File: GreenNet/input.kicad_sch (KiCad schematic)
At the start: 74 parts, among them Q3 IRF9358TRPBF, Q4 SI3932DV-T1-GE3, Q5 SI3993CDV-T1-GE3, U2 USB_C_Receptacle_12P, U3 USB_C_Receptacle_12P, U4 CP2102N-A02-GQFN28, U6 CYPD3177-24LQXQT

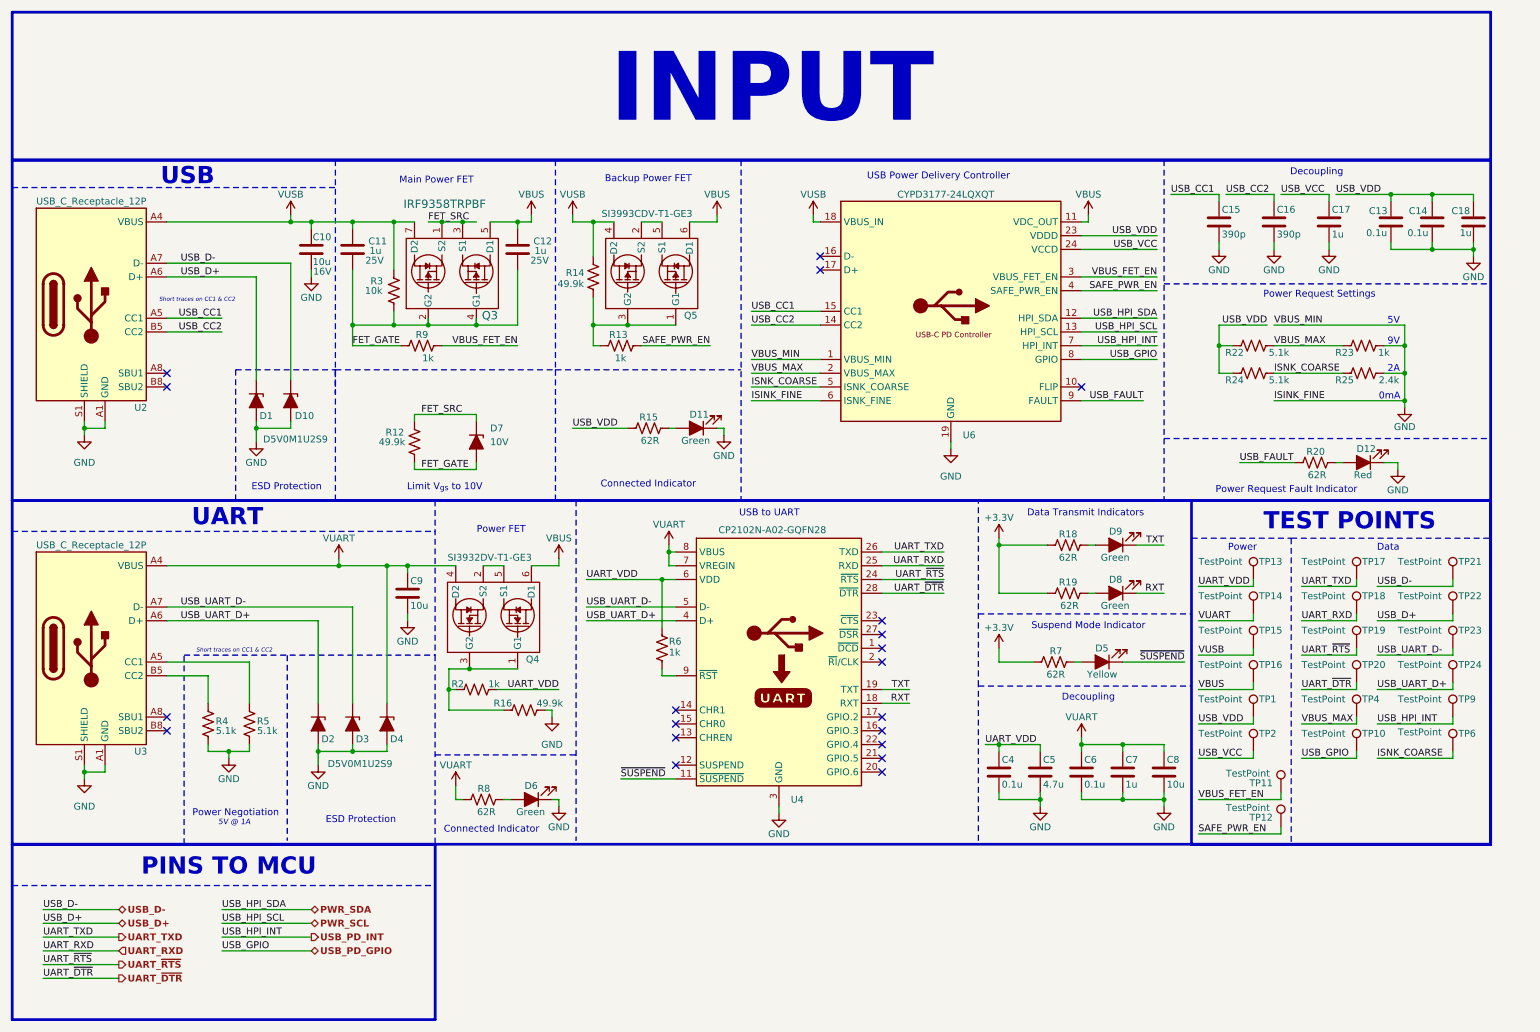
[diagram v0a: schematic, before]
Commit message: update
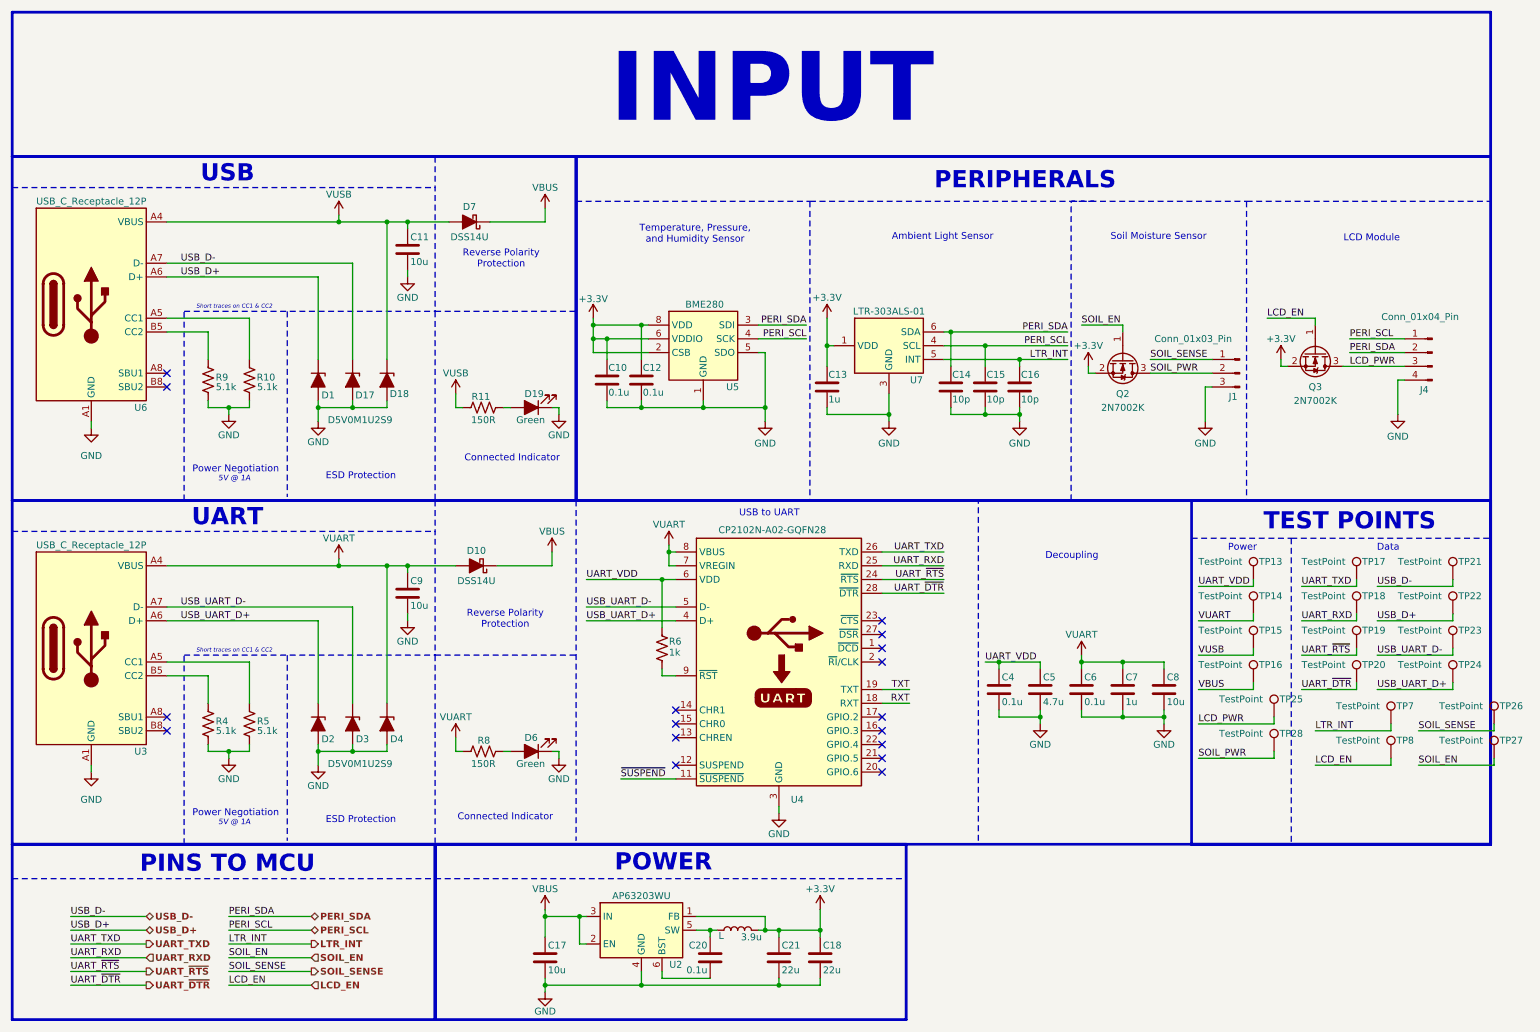
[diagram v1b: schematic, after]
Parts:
- removed D10: D5V0M1U2S9, AA_Diodes:D5V0M1U2S9Q, symbol Device:D_Zener_Filled
- removed D11, D8, D9: Green, LED_SMD:LED_0805_2012Metric, symbol Device:LED_Filled
- removed D12: Red, LED_SMD:LED_0805_2012Metric, symbol Device:LED_Filled
- removed D5: Yellow, LED_SMD:LED_0805_2012Metric, symbol Device:LED_Filled
- removed D7: 10V, AA_Diodes:NHZ10C,115, symbol Device:D_Zener_Filled
- removed Q3: IRF9358TRPBF, AA_FETS:SO8_IRF9358TRPBF_INF, symbol AA_FETs:IRF9358TRPBF
- removed Q4: SI3932DV-T1-GE3, AA_FETS:TSOP_0DV-T1-E3_VIS, symbol AA_FETs:SI3932DV-T1-GE3
- removed Q5: SI3993CDV-T1-GE3, AA_FETS:TSOP_0DV-T1-E3_VIS, symbol AA_FETs:SI3993CDV-T1-GE3
- removed R12, R14, R16: 49.9k, Resistor_SMD:R_0805_2012Metric, symbol Device:R_US
- removed R13, R2, R23: 1k, Resistor_SMD:R_0805_2012Metric, symbol Device:R_US
- removed R15, R18, R19, R20, R7: 62R, Resistor_SMD:R_0805_2012Metric, symbol Device:R_US
- removed R22, R24: 5.1k, Resistor_SMD:R_0805_2012Metric, symbol Device:R_US
- removed R25: 2.4k, Resistor_SMD:R_0805_2012Metric, symbol Device:R_US
- removed R3: 10k, Resistor_SMD:R_0805_2012Metric, symbol Device:R_US
- removed TP1, TP10, TP11, TP12, TP2, TP4, TP6, TP9: TestPoint, AA_TestPoints:RCWCTE, symbol Connector:TestPoint
- removed U2: USB_C_Receptacle_12P, AA_Connectors:GCT_USB4105-GF-A, symbol AA_Connectors:USB_C_Receptacle_12P
- removed U6: CYPD3177-24LQXQT, AA_Interface_USB:QFN50P400X400X60-25N-D, symbol AA_Interface_USB:CYPD3177-24LQXQT
- added 3.9u: L, symbol Device:L
- added C20: 0.1u, Capacitor_SMD:C_0805_2012Metric, symbol Device:C
- added C21: 22u, Capacitor_SMD:C_0805_2012Metric, symbol Device:C
- added D10, D7: DSS14U, symbol Device:D_Schottky_Filled
- added D17, D18: D5V0M1U2S9, AA_Diodes:D5V0M1U2S9Q, symbol Device:D_Zener_Filled
- added D19: Green, LED_SMD:LED_0805_2012Metric, symbol Device:LED_Filled
- added J1: Conn_01x03_Pin, AA_Connectors:61300311121, symbol Connector:Conn_01x03_Pin
- added J4: Conn_01x04_Pin, AA_Connectors:61300411121, symbol Connector:Conn_01x04_Pin
- added Q2, Q3: 2N7002K, Package_TO_SOT_SMD:SOT-23, symbol Transistor_FET:2N7002K
- added R10: 5.1k, Resistor_SMD:R_0805_2012Metric, symbol Device:R_US
- added R11: 150R, Resistor_SMD:R_0805_2012Metric, symbol Device:R_US
- added TP25, TP26, TP27, TP28, TP7, TP8: TestPoint, AA_TestPoints:RCWCTE, symbol Connector:TestPoint
- added U2: AP63203WU, Package_TO_SOT_SMD:TSOT-23-6, symbol Regulator_Switching:AP63203WU
- added U5: BME280, Package_LGA:Bosch_LGA-8_2.5x2.5mm_P0.65mm_ClockwisePinNumbering, symbol Sensor:BME280
- added U6: USB_C_Receptacle_12P, AA_Connectors:GCT_USB4105-GF-A, symbol AA_Connectors:USB_C_Receptacle_12P
- added U7: LTR-303ALS-01, OptoDevice:Lite-On_LTR-303ALS-01, symbol Sensor_Optical:LTR-303ALS-01
- C10: value 10u -> 0.1u
- C11, C17: value 1u -> 10u
- C12: value 1u -> 0.1u
- C13: value 0.1u -> 1u
- C14: value 0.1u -> 10p
- C15, C16: value 390p -> 10p
- C18: value 1u -> 22u
- R8: value 62R -> 150R
- R9: value 1k -> 5.1k
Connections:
- net USB_VCC is gone; now on net VBUS: C17.1
- net +3.3V: now also C10.1, C12.1, C13.1, C18.1, 3.9u.2, C21.1, Q2.2 (S), Q3.2 (S), U2.1 (FB), U5.2 (CSB), U5.6 (VDDIO), U5.8 (VDD), U7.1 (VDD)
- net USB_D+: now also U6.A6 (D+), U6.B6 (D+)
- net USB_D-: now also D17.1 (K), U6.A7 (D-), U6.B7 (D-)
- net VBUS: now also D10.1 (K), D7.1 (K), U2.2 (EN), U2.3 (IN); no longer C12.2
- net VUART: now also D10.2 (A)
- net VUSB: now also C11.1, D18.1 (K), D7.2 (A), R11.1, U6.A4 (VBUS), U6.B4 (VBUS); no longer C10.1, C11.2
- net EP renamed GND
- net GND: now also C11.2, C12.2, R9.1, C21.2, D17.2 (A), D18.2 (A), D19.1 (K), J1.3 (Pin_3), J4.4 (Pin_4), R10.1, U2.4 (GND), U5.1 (GND), U5.5 (SDO), U5.7 (GND), U6.A1 (GND), U6.B1 (GND), U6.S1 (SHIELD), U7.3 (GND)
- removed net FET_GATE: C11.1, C12.1, R9.1
- net USB_CC1 renamed PERI_SCL
- net PERI_SCL: now also J4.1 (Pin_1), U5.4 (SCK), U7.4 (SCL)
- net USB_CC2 renamed LTR_INT
- net LTR_INT: now also TP7.1, U7.5 (INT)
- removed net USB_VDD: C13.1, C14.1, C18.1
- net VBUS_FET_EN: no longer names the net of R9.2
- net VBUS_FET_EN: now also U6.B5 (CC2)
- new net: 3.9u.1, C20.1, U2.5 (SW)
- new net: D19.2 (A), R11.2
- new net: C20.2, U2.6 (BST)
- new net: R10.2, U6.A5 (CC1)
- new net LCD_EN: Q3.1 (G), TP8.1
- new net LCD_PWR: J4.3 (Pin_3), Q3.3 (D), TP25.1
- new net PERI_SDA: C14.1, J4.2 (Pin_2), U5.3 (SDI), U7.6 (SDA)
- new net SOIL_EN: Q2.1 (G), TP27.1
- new net SOIL_PWR: J1.2 (Pin_2), Q2.3 (D), TP28.1
- new net SOIL_SENSE: J1.1 (Pin_1), TP26.1
- no-connect marks 20 -> 17
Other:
- note added: "Ambient Light Sensor"
- note added: "LCD Module"
- note added: "PERIPHERALS"
- note added: "POWER"
- note added: "Reverse Polarity Protection"
- note added: "Soil Moisture Sensor"
- note added: "Temperature, Pressure, and Humidity Sensor"
- note removed: "0mA"
- note removed: "2A"
- note removed: "5V"
- note removed: "9V"
- note removed: "Backup Power FET"
- note removed: "Data Transmit Indicators"
- note removed: "Limit V_{gs} to 10V"
- note removed: "Main Power FET"
- note removed: "Power FET"
- note removed: "Power Request Fault Indicator"
- note removed: "Power Request Settings"
- note removed: "Suspend Mode Indicator"
- note removed: "USB Power Delivery Controller"
- moved on the sheet: C4, C5, C6, C7, C8, D6, R8
